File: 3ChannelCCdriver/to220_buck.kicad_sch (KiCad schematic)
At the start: 10 parts, among them U4 TPS54202DDC

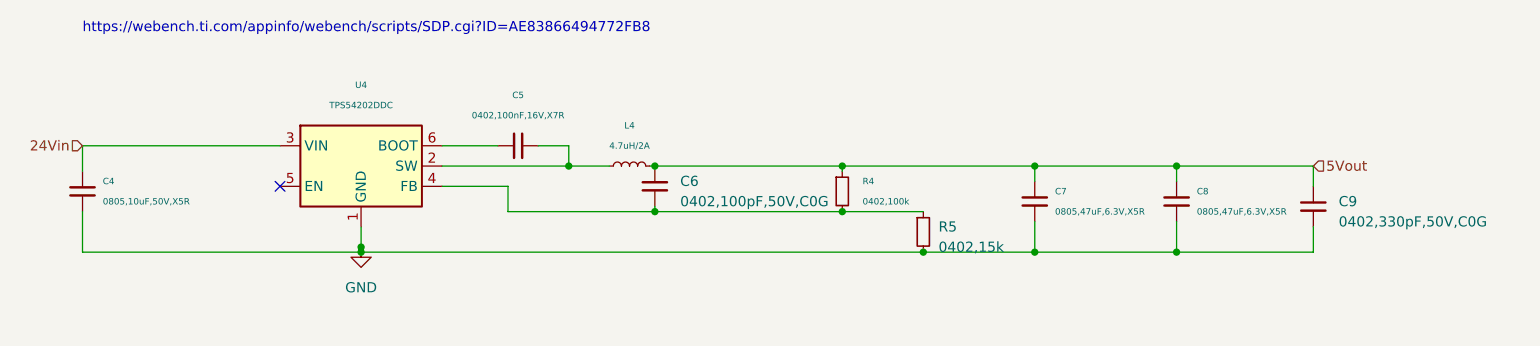
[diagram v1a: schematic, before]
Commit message: neat-ified schematics
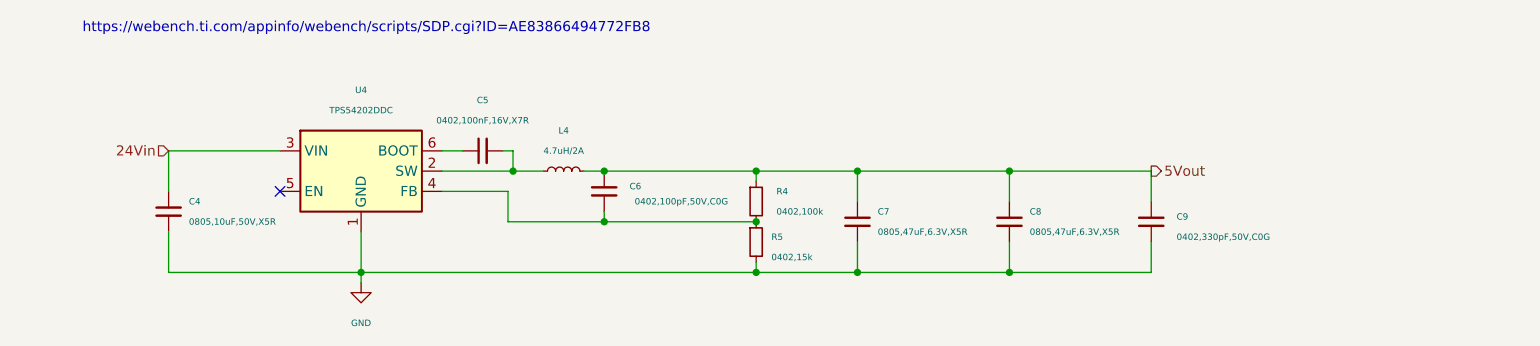
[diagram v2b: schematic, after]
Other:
- title: (none) -> 24V to 5V Buck
- moved on the sheet: C4, C5, C6, C7, C8, C9, L4, R4, R5, U4
